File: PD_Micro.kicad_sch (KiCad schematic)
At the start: 43 parts, among them J1 Conn_01x02, Q1 DMP3017SFK, Q2 DTC143E, SW1 SW_DIP_x06, SW2 SW_DPST_x2, SW3 SW_Push, SW4 SW_Push, SW5 SW_DPST_x2, U1 SRV05-4, U2 Pico, U3 TPS62175DQC, U4 FUSB302BMPX, U5 ACS723xLCTR-10AB, U6 oledSym

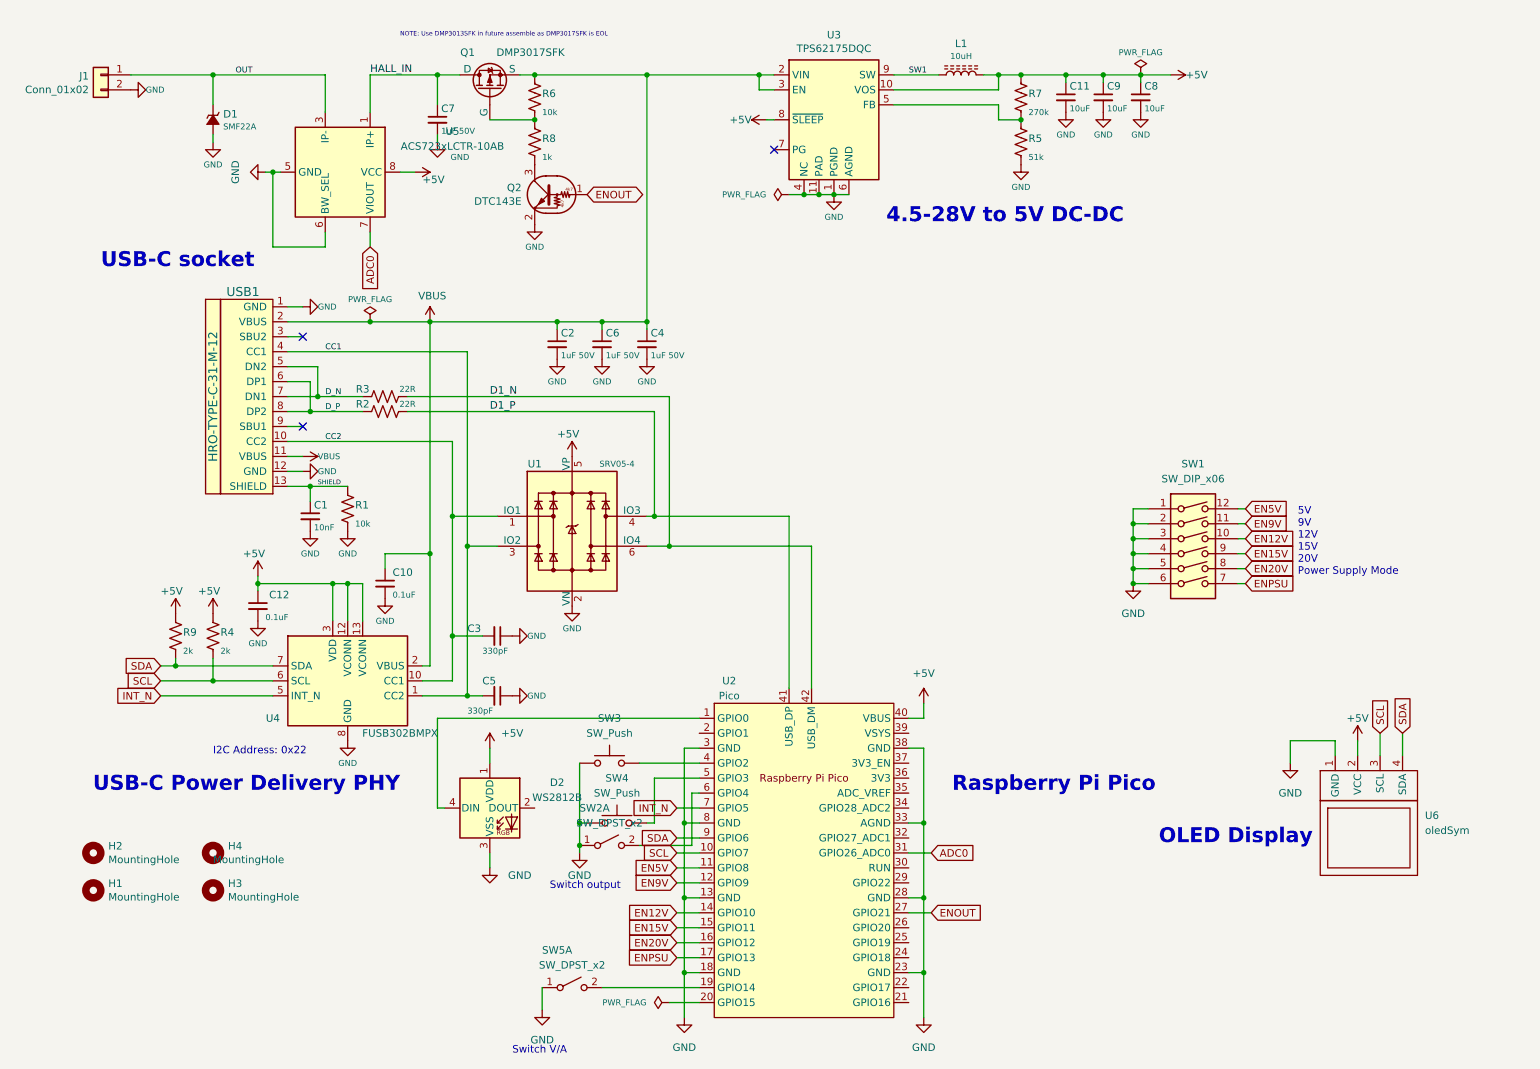
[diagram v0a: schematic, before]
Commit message: schematic finished
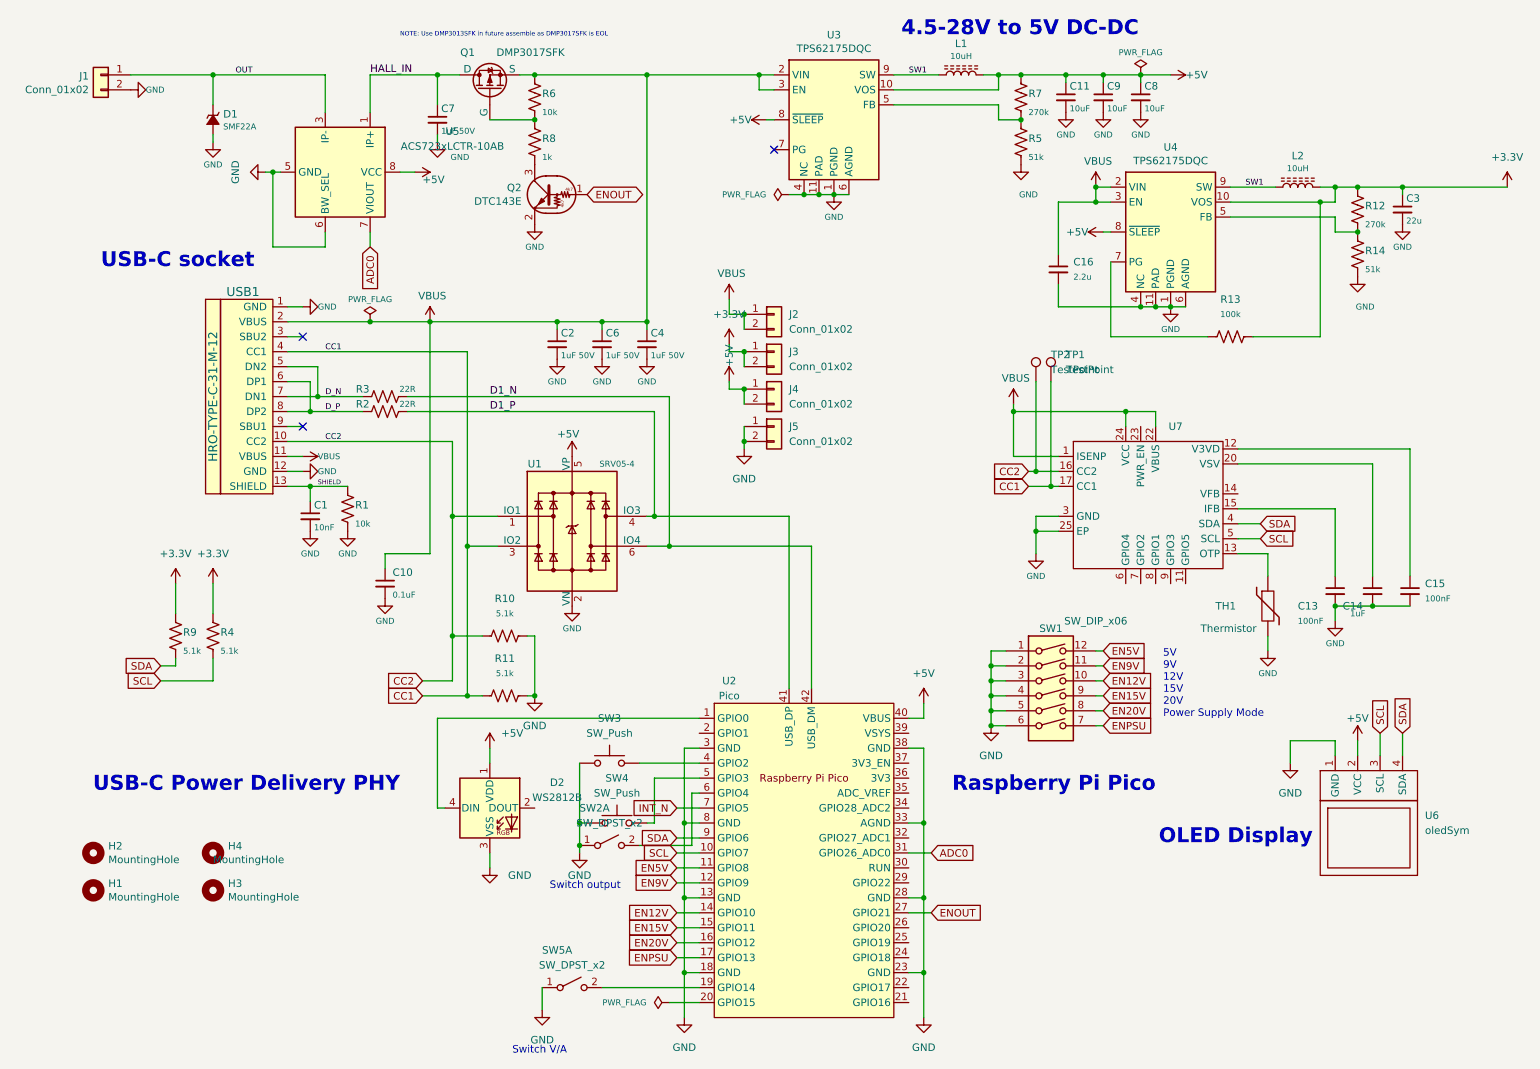
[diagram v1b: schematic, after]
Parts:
- removed C12: 0.1uF, Capacitor_SMD:C_0805_2012Metric, symbol -Passive:C
- removed C5: 330pF, Capacitor_SMD:C_0805_2012Metric, symbol -Passive:C
- removed U4: FUSB302BMPX, -Chip:WQFN-14-1EP_2.5x2.5mm_P0.5mm_EP1.45x1.45mm, symbol -Chip:FUSB302BMPX
- added C13: 100nF, Package_DFN_QFN:WQFN-24-1EP_4x4mm_P0.5mm_EP2.6x2.6mm, symbol -Passive:C
- added C14: 1uF, Capacitor_SMD:C_0805_2012Metric, symbol -Passive:C
- added C15: 100nF, Capacitor_SMD:C_0805_2012Metric, symbol -Passive:C
- added C16: 2.2u, Capacitor_SMD:C_0805_2012Metric, symbol -Passive:C
- added J2, J3, J4, J5: Conn_01x02, symbol -Connector:Conn_01x02
- added L2: 10uH, -Passive:L_4012, symbol -Passive:L_cored
- added R10, R11: 5.1k, symbol -Passive:R
- added R12: 270k, Resistor_SMD:R_0805_2012Metric, symbol -Passive:R
- added R13: 100k, symbol -Passive:R
- added R14: 51k, Resistor_SMD:R_0805_2012Metric, symbol -Passive:R
- added TH1: Thermistor, symbol Device:Thermistor
- added TP1, TP2: TestPoint, symbol -Connector:TestPoint
- added U4: TPS62175DQC, -Chip:WSON-10-1EP_2x3mm_P0.5mm_EP0.84x2.4mm, symbol -Chip:TPS62175DQC
- added U7: ~, Package_DFN_QFN:WQFN-24-1EP_4x4mm_P0.5mm_EP2.6x2.6mm, symbol AP33772:AP33772
- C3: value 330pF -> 22u
- R4, R9: value 2k -> 5.1k
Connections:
- net +5V: now also J4.1 (Pin_1), J4.2 (Pin_2), U4.8 (~{SLEEP}); no longer R4.1, R9.1
- net CC1: now also R11.1, TP1.1, U7.17 (CC1)
- net CC2: now also R10.1, TP2.1, U7.16 (CC2); no longer C3.2
- net GND: now also C3.2, C13.2, C14.2, C15.2, C16.2, J5.1 (Pin_1), J5.2 (Pin_2), R10.2, R11.2, R14.2, TH1.2, U4.1 (PGND), U4.11 (PAD), U4.4 (NC), U4.6 (AGND), U7.25 (EP), U7.3 (GND); no longer C3.1
- net SCL: now also U7.5 (SCL)
- net SDA: now also U7.4 (SDA)
- net SW1: now also L2.1, U4.9 (SW)
- net VBUS: now also C16.1, J2.1 (Pin_1), J2.2 (Pin_2), U4.2 (VIN), U4.3 (EN), U7.1 (ISENP), U7.22 (VBUS), U7.24 (VCC)
- new net: R13.1, U4.7 (PG)
- new net: R12.2, R14.1, U4.5 (FB)
- new net: C14.1, U7.20 (VSV)
- new net: C13.1, U7.15 (IFB)
- new net: C15.1, U7.12 (V3VD)
- new net: TH1.1, U7.13 (OTP)
- new net +3.3V: C3.1, J3.1 (Pin_1), J3.2 (Pin_2), L2.2, R12.1, R13.2, R4.1, R9.1, U4.10 (VOS)
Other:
- note removed: "I2C Address: 0x22"
- moved on the sheet: SW1
